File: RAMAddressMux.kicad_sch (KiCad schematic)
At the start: 18 parts, among them J1 74LS257

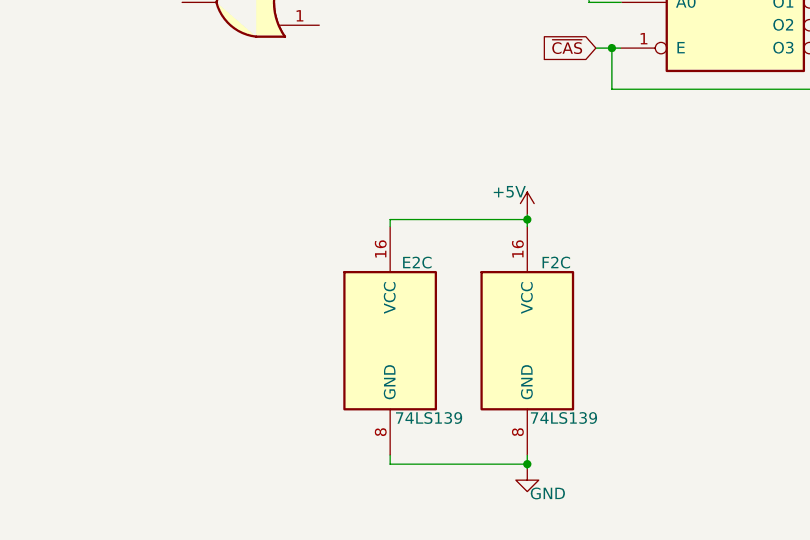
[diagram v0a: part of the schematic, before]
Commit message: Add files via upload
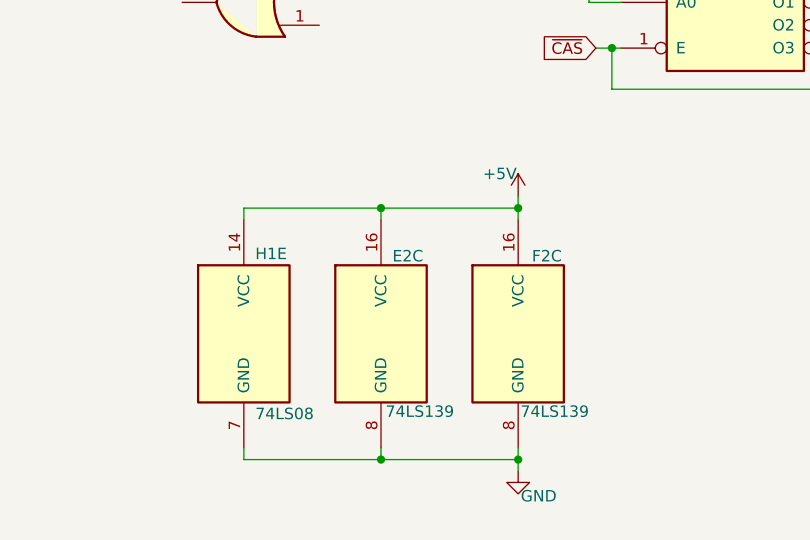
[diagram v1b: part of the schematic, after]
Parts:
- added unit 5 of H1
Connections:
- net +5V: now also H1.14 (VCC)
- net GND: now also H1.7 (GND)
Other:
- moved on the sheet: E2C, F2C
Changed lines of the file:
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@@
   (junction (at 300.482 140.97) (diameter 0) (color 0 0 0 0)
   )
+  (junction (at 212.09 223.52) (diameter 0) (color 0 0 0 0)
+  )
   (junction (at 273.05 111.76) (diameter 0) (color 0 0 0 0)
   )
-  (junction (at 228.346 224.028) (diameter 0) (color 0 0 0 0)
-  )
   (junction (at 237.744 177.8) (diameter 0) (color 0 0 0 0)
   )
@@
   (junction (at 230.378 111.76) (diameter 0) (color 0 0 0 0)
   )
+  (junction (at 227.33 195.58) (diameter 0) (color 0 0 0 0)
+  )
   (junction (at 236.982 152.4) (diameter 0) (color 0 0 0 0)
   )
@@
   (junction (at 266.954 104.14) (diameter 0) (color 0 0 0 0)
   )
+  (junction (at 212.09 195.58) (diameter 0) (color 0 0 0 0)
+  )
   (junction (at 297.942 135.89) (diameter 0) (color 0 0 0 0)
   )
@@
   (junction (at 235.204 154.94) (diameter 0) (color 0 0 0 0)
   )
-  (junction (at 228.346 196.85) (diameter 0) (color 0 0 0 0)
-  )
   (junction (at 319.532 96.012) (diameter 0) (color 0 0 0 0)
   )
   (junction (at 236.982 122.936) (diameter 0) (color 0 0 0 0)
+  )
+  (junction (at 227.33 223.52) (diameter 0) (color 0 0 0 0)
   )
   (no_connect (at 110.236 171.196))
@@
     (stroke (width 0) (type default))
   )
-  (wire (pts (xy 228.346 224.536) (xy 228.346 224.028))
+  (wire (pts (xy 227.33 223.52) (xy 227.33 224.79))
     (stroke (width 0) (type default))
   )
@@
     (stroke (width 0) (type default))
   )
-  (wire (pts (xy 213.106 196.85) (xy 228.346 196.85))
+  (wire (pts (xy 212.09 195.58) (xy 227.33 195.58))
     (stroke (width 0) (type default))
   )
@@
     (stroke (width 0) (type default))
   )
-  (wire (pts (xy 228.346 224.028) (xy 228.346 223.012))
-    (stroke (width 0) (type default))
-  )
   (wire (pts (xy 110.236 166.116) (xy 119.126 166.116))
     (stroke (width 0) (type default))
@@
     (stroke (width 0) (type default))
   )
-  (wire (pts (xy 213.106 224.028) (xy 228.346 224.028))
+  (wire (pts (xy 196.85 223.52) (xy 212.09 223.52))
     (stroke (width 0) (type default))
   )
@@
     (stroke (width 0) (type default))
   )
-  (wire (pts (xy 213.106 197.612) (xy 213.106 196.85))
+  (wire (pts (xy 212.09 195.58) (xy 212.09 196.85))
     (stroke (width 0) (type default))
   )
@@
     (stroke (width 0) (type default))
   )
+  (wire (pts (xy 227.33 194.31) (xy 227.33 195.58))
+    (stroke (width 0) (type default))
+  )
   (wire (pts (xy 213.36 104.14) (xy 238.76 104.14))
     (stroke (width 0) (type default))
   )
-  (wire (pts (xy 213.106 223.012) (xy 213.106 224.028))
+  (wire (pts (xy 227.33 222.25) (xy 227.33 223.52))
+    (stroke (width 0) (type default))
+  )
+  (wire (pts (xy 212.09 222.25) (xy 212.09 223.52))
     (stroke (width 0) (type default))
   )
@@
     (stroke (width 0) (type default))
   )
+  (wire (pts (xy 212.09 195.58) (xy 196.85 195.58))
+    (stroke (width 0) (type default))
+  )
   (wire (pts (xy 84.836 178.816) (xy 81.026 178.816))
     (stroke (width 0) (type default))
@@
     (stroke (width 0) (type default))
   )
+  (wire (pts (xy 212.09 223.52) (xy 227.33 223.52))
+    (stroke (width 0) (type default))
+  )
   (wire (pts (xy 81.28 176.276) (xy 84.836 176.276))
     (stroke (width 0) (type default))
@@
     (stroke (width 0) (type default))
   )
+  (wire (pts (xy 196.85 195.58) (xy 196.85 196.85))
+    (stroke (width 0) (type default))
+  )
   (wire (pts (xy 82.804 75.946) (xy 82.804 47.752))
     (stroke (width 0) (type default))
@@
     (stroke (width 0) (type default))
   )
-  (wire (pts (xy 228.346 196.342) (xy 228.346 196.85))
-    (stroke (width 0) (type default))
-  )
   (wire (pts (xy 287.274 192.532) (xy 291.338 192.532))
     (stroke (width 0) (type default))
@@
     (stroke (width 0) (type default))
   )
-  (wire (pts (xy 228.346 196.85) (xy 228.346 197.612))
+  (wire (pts (xy 227.33 195.58) (xy 227.33 196.85))
     (stroke (width 0) (type default))
   )
@@
   )
   (wire (pts (xy 144.78 171.196) (xy 144.78 172.212))
+    (stroke (width 0) (type default))
+  )
+  (wire (pts (xy 196.85 222.25) (xy 196.85 223.52))
     (stroke (width 0) (type default))
   )
@@
     )
   )
-  (symbol (lib_id "74xx:74LS139") (at 228.346 210.312 0) (unit 3)
-    (in_bom yes) (on_board yes) (dnp no)
-    (property "Reference" "F2" (at 229.87 201.676 0)
+  (symbol (lib_id "74xx:74LS139") (at 227.33 209.55 0) (unit 3)
+    (in_bom yes) (on_board yes) (dnp no)
+    (property "Reference" "F2" (at 228.854 200.914 0)
       (effects (font (size 1.27 1.27)) (justify left))
     )
-    (property "Value" "74LS139" (at 228.6 218.948 0)
+    (property "Value" "74LS139" (at 227.584 218.186 0)
       (effects (font (size 1.27 1.27)) (justify left))
     )
-    (property "Footprint" "Apple:DIP-16_W7.62mm" (at 228.346 210.312 0)
-      (effects (font (size 1.27 1.27)) hide)
-    )
-    (property "Datasheet" "http://www.ti.com/lit/ds/symlink/sn74ls139a.pdf" (at 228.346 210.312 0)
+    (property "Footprint" "Apple:DIP-16_W7.62mm" (at 227.33 209.55 0)
+      (effects (font (size 1.27 1.27)) hide)
+    )
+    (property "Datasheet" "http://www.ti.com/lit/ds/symlink/sn74ls139a.pdf" (at 227.33 209.55 0)
       (effects (font (size 1.27 1.27)) hide)
     )
@@
     )
   )
-  (symbol (lib_id "74xx:74LS139") (at 213.106 210.312 0) (unit 3)
-    (in_bom yes) (on_board yes) (dnp no)
-    (property "Reference" "E2" (at 214.376 201.676 0)
+  (symbol (lib_id "74xx:74LS139") (at 212.09 209.55 0) (unit 3)
+    (in_bom yes) (on_board yes) (dnp no)
+    (property "Reference" "E2" (at 213.36 200.914 0)
       (effects (font (size 1.27 1.27)) (justify left))
     )
-    (property "Value" "74LS139" (at 213.614 218.948 0)
+    (property "Value" "74LS139" (at 212.598 218.186 0)
       (effects (font (size 1.27 1.27)) (justify left))
     )
-    (property "Footprint" "Apple:DIP-16_W7.62mm" (at 213.106 210.312 0)
-      (effects (font (size 1.27 1.27)) hide)
-    )
-    (property "Datasheet" "http://www.ti.com/lit/ds/symlink/sn74ls139a.pdf" (at 213.106 210.312 0)
+    (property "Footprint" "Apple:DIP-16_W7.62mm" (at 212.09 209.55 0)
+      (effects (font (size 1.27 1.27)) hide)
+    )
+    (property "Datasheet" "http://www.ti.com/lit/ds/symlink/sn74ls139a.pdf" (at 212.09 209.55 0)
       (effects (font (size 1.27 1.27)) hide)
     )
@@
     )
   )
-  (symbol (lib_id "power:+5V") (at 228.346 196.342 0) (unit 1)
-    (in_bom yes) (on_board yes) (dnp no)
-    (property "Reference" "#PWR0284" (at 228.346 200.152 0)
-      (effects (font (size 1.27 1.27)) hide)
-    )
-    (property "Value" "+5V" (at 226.314 193.802 0)
-      (effects (font (size 1.27 1.27)))
-    )
-    (property "Footprint" "" (at 228.346 196.342 0)
-      (effects (font (size 1.27 1.27)) hide)
-    )
-    (property "Datasheet" "" (at 228.346 196.342 0)
+  (symbol (lib_id "power:+5V") (at 227.33 194.31 0) (unit 1)
+    (in_bom yes) (on_board yes) (dnp no)
+    (property "Reference" "#PWR0284" (at 227.33 198.12 0)
+      (effects (font (size 1.27 1.27)) hide)
+    )
+    (property "Value" "+5V" (at 225.298 191.77 0)
+      (effects (font (size 1.27 1.27)))
+    )
+    (property "Footprint" "" (at 227.33 194.31 0)
+      (effects (font (size 1.27 1.27)) hide)
+    )
+    (property "Datasheet" "" (at 227.33 194.31 0)
       (effects (font (size 1.27 1.27)) hide)
     )
@@
     )
   )
-  (symbol (lib_id "power:GND") (at 228.346 224.536 0) (unit 1)
-    (in_bom yes) (on_board yes) (dnp no)
-    (property "Reference" "#PWR0285" (at 228.346 230.886 0)
-      (effects (font (size 1.27 1.27)) hide)
-    )
-    (property "Value" "GND" (at 230.632 227.33 0)
-      (effects (font (size 1.27 1.27)))
-    )
-    (property "Footprint" "" (at 228.346 224.536 0)
-      (effects (font (size 1.27 1.27)) hide)
-    )
-    (property "Datasheet" "" (at 228.346 224.536 0)
+  (symbol (lib_id "power:GND") (at 227.33 224.79 0) (unit 1)
+    (in_bom yes) (on_board yes) (dnp no)
+    (property "Reference" "#PWR0285" (at 227.33 231.14 0)
+      (effects (font (size 1.27 1.27)) hide)
+    )
+    (property "Value" "GND" (at 229.616 227.584 0)
+      (effects (font (size 1.27 1.27)))
+    )
+    (property "Footprint" "" (at 227.33 224.79 0)
+      (effects (font (size 1.27 1.27)) hide)
+    )
+    (property "Datasheet" "" (at 227.33 224.79 0)
       (effects (font (size 1.27 1.27)) hide)
     )
@@
         )
       )
+    )
+  )
+  (symbol (lib_id "74xx:74LS08") (at 196.85 209.55 0) (unit 5)
+    (in_bom yes) (on_board yes) (dnp no)
+    (property "Reference" "H1" (at 198.12 200.66 0)
+      (effects (font (size 1.27 1.27)) (justify left))
+    )
+    (property "Value" "74LS08" (at 198.12 218.44 0)
+      (effects (font (size 1.27 1.27)) (justify left))
+    )
+    (property "Footprint" "" (at 196.85 209.55 0)
+      (effects (font (size 1.27 1.27)) hide)
+    )
+    (property "Datasheet" "http://www.ti.com/lit/gpn/sn74LS08" (at 196.85 209.55 0)
+      (effects (font (size 1.27 1.27)) hide)
+    )
+    (pin "14")
+    (pin "7")
+    (pin "5")
+    (pin "11")
+    (pin "13")
+    (pin "4")
+    (pin "8")
+    (pin "9")
+    (pin "6")
+    (pin "1")
+    (pin "2")
+    (pin "3")
+    (pin "12")
+    (pin "10")
+    (instances
+      (project "AppleII"
+        (path "/f1f08369-4db3-46f7-9b89-a5d3cfbed55a/00000000-0000-0000-0000-000060210f9e"
+          (reference "H1") (unit 5)
+        )
+      )
